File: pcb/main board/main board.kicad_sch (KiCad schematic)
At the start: 36 parts, among them J10 12V Battery, J11 BAU, J12 Servo 4 Conn, J13 Servo 1 Conn, J14 Servo 2 Conn, J15 Servo 3 Conn, J16 Servo 5 Conn, J17 Servo 6 Conn, J18 Servo 7 Conn, J19 Servo 8 Conn, J5 I2C 0 Conn, J6 I2C 1 Conn, Q1 IRF8714PBF, Q2 IRF8714PBF, U4 MCP23017_SO, U6 LM3150MH

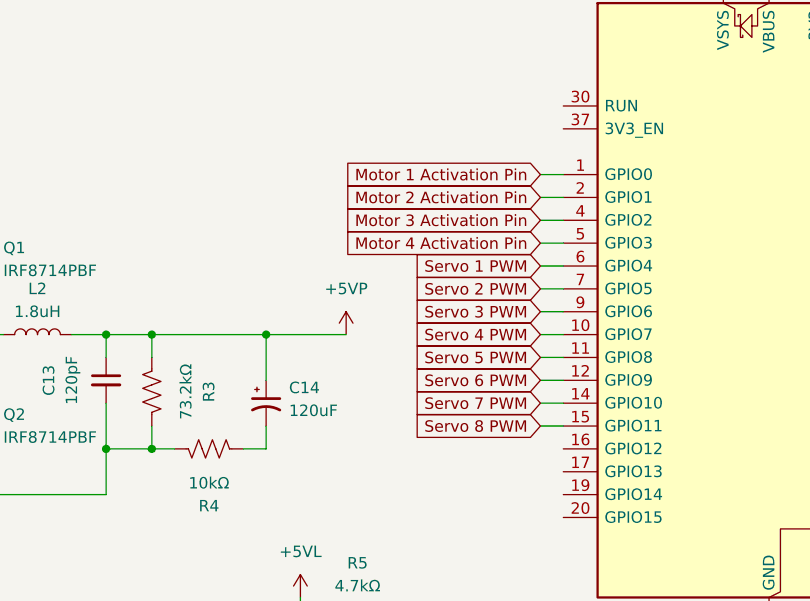
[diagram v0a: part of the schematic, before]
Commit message: Almost finished PCB !
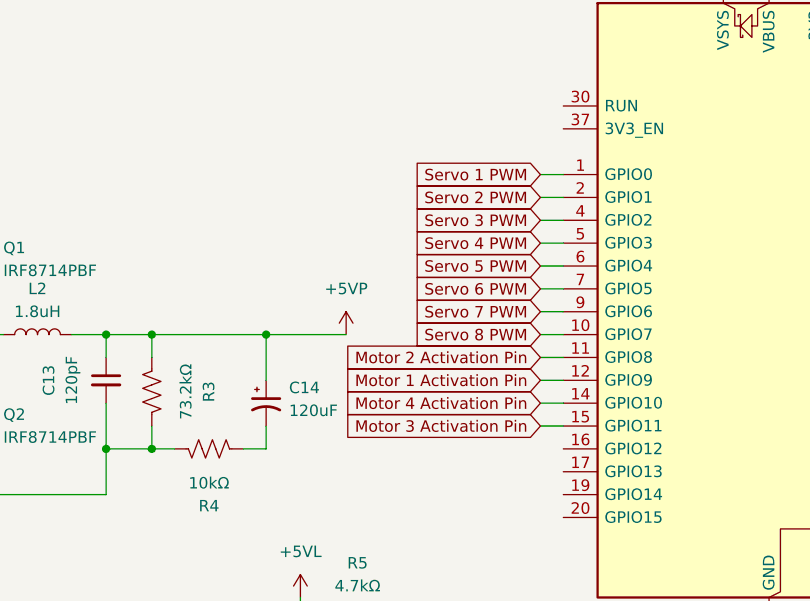
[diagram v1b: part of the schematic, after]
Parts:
- A1, A2: footprint Module:RaspberryPi_Pico_Common_Unspecified -> Module:RaspberryPi_Pico_Common_THT
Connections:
- net Motor 1 Activation Pin: now also A1.12 (GPIO9); no longer A1.1 (GPIO0)
- net Motor 2 Activation Pin: now also A1.11 (GPIO8); no longer A1.2 (GPIO1)
- net Motor 3 Activation Pin: now also A1.15 (GPIO11); no longer A1.4 (GPIO2)
- net Motor 4 Activation Pin: now also A1.14 (GPIO10); no longer A1.5 (GPIO3)
- net Servo 1 PWM: now also A1.1 (GPIO0); no longer A1.6 (GPIO4)
- net Servo 2 PWM: now also A1.2 (GPIO1); no longer A1.7 (GPIO5)
- net Servo 3 PWM: now also A1.4 (GPIO2); no longer A1.9 (GPIO6)
- net Servo 4 PWM: now also A1.5 (GPIO3); no longer A1.10 (GPIO7)
- net Servo 5 PWM: now also A1.6 (GPIO4); no longer A1.11 (GPIO8)
- net Servo 6 PWM: now also A1.7 (GPIO5); no longer A1.12 (GPIO9)
- net Servo 7 PWM: now also A1.9 (GPIO6); no longer A1.14 (GPIO10)
- net Servo 8 PWM: now also A1.10 (GPIO7); no longer A1.15 (GPIO11)
